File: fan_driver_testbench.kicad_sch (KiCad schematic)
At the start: 6 parts, among them Q5 BTS141

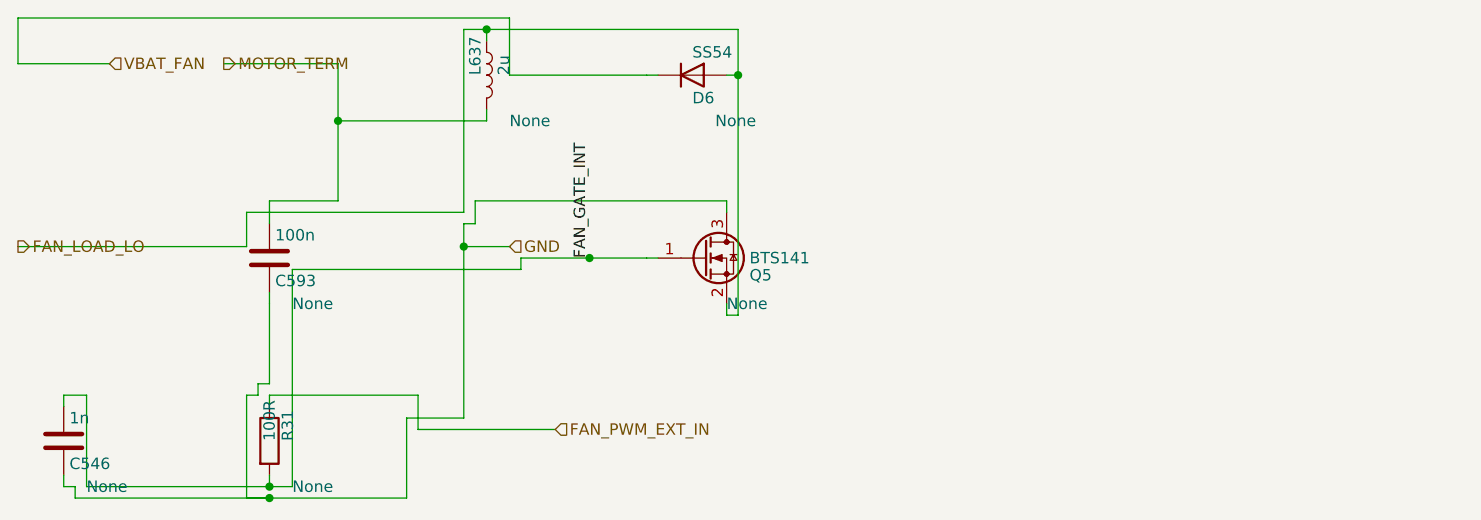
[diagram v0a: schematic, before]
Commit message: refactoring
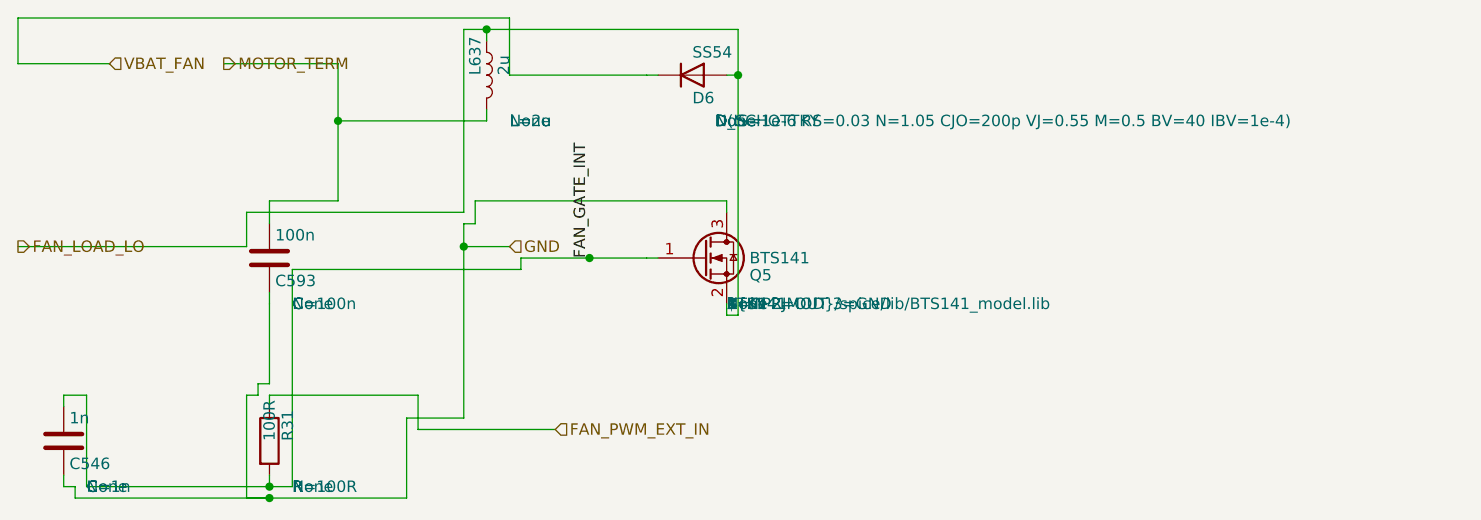
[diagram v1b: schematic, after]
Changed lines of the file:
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@@
+			)
+		)
+		(property "Sim.Device" "R"
+			(at 34.29 53.3399 0)
+			(effects
+				(font
+					(size 1.27 1.27)
+				)
+				(justify left)
+			)
+		)
+		(property "Sim.Params" "R=100R"
+			(at 34.29 53.3399 0)
+			(effects
+				(font
+					(size 1.27 1.27)
+				)
+				(justify left)
 			)
 		)
@@
 		(instances
 			(project "climate_control_niva_travel"
-				(path "/769b9906-d389-4980-b175-619cd77c101f"
+				(path "/04e9baa8-05c1-4d46-8e7f-66f0ccb7f2e0"
 					(reference "R31")
 					(unit 1)
@@
 			)
 		)
+		(property "Sim.Device" "C"
+			(at 11.43 53.3399 0)
+			(effects
+				(font
+					(size 1.27 1.27)
+				)
+				(justify left)
+			)
+		)
+		(property "Sim.Params" "C=1n"
+			(at 11.43 53.3399 0)
+			(effects
+				(font
+					(size 1.27 1.27)
+				)
+				(justify left)
+			)
+		)
 		(pin "1"
 		)
@@
 		(instances
 			(project "climate_control_niva_travel"
-				(path "/769b9906-d389-4980-b175-619cd77c101f"
+				(path "/04e9baa8-05c1-4d46-8e7f-66f0ccb7f2e0"
 					(reference "C546")
 					(unit 1)
@@
 			)
 		)
+		(property "Sim.Device" "X"
+			(at 82.55 33.0199 0)
+			(effects
+				(font
+					(size 1.27 1.27)
+				)
+				(justify left)
+			)
+		)
+		(property "Sim.Name" "BTS141"
+			(at 82.55 33.0199 0)
+			(effects
+				(font
+					(size 1.27 1.27)
+				)
+				(justify left)
+			)
+		)
+		(property "Sim.Library" "${KIPRJMOD}/spice/lib/BTS141_model.lib"
+			(at 82.55 33.0199 0)
+			(effects
+				(font
+					(size 1.27 1.27)
+				)
+				(justify left)
+			)
+		)
+		(property "Sim.Pins" "1=IN 2=OUT 3=GND"
+			(at 82.55 33.0199 0)
+			(effects
+				(font
+					(size 1.27 1.27)
+				)
+				(justify left)
+			)
+		)
+		(property "Sim.Enable" "1"
+			(at 82.55 33.0199 0)
+			(effects
+				(font
+					(size 1.27 1.27)
+				)
+				(justify left)
+			)
+		)
 		(pin "1"
 		)
@@
 		(instances
 			(project "climate_control_niva_travel"
-				(path "/769b9906-d389-4980-b175-619cd77c101f"
+				(path "/04e9baa8-05c1-4d46-8e7f-66f0ccb7f2e0"
 					(reference "Q5")
 					(unit 1)
@@
 			)
 		)
+		(property "Sim.Device" "D"
+			(at 81.28 12.6999 0)
+			(effects
+				(font
+					(size 1.27 1.27)
+				)
+				(justify left)
+			)
+		)
+		(property "Sim.Model" "D_SCHOTTKY"
+			(at 81.28 12.6999 0)
+			(effects
+				(font
+					(size 1.27 1.27)
+				)
+				(justify left)
+			)
+		)
+		(property "Sim.Params" "D(IS=1e-6 RS=0.03 N=1.05 CJO=200p VJ=0.55 M=0.5 BV=40 IBV=1e-4)"
+			(at 81.28 12.6999 0)
+			(effects
+				(font
+					(size 1.27 1.27)
+				)
+				(justify left)
+			)
+		)
 		(pin "1"
 		)
@@
 		(instances
 			(project "climate_control_niva_travel"
-				(path "/769b9906-d389-4980-b175-619cd77c101f"
+				(path "/04e9baa8-05c1-4d46-8e7f-66f0ccb7f2e0"
 					(reference "D6")
 					(unit 1)
@@
 			)
 		)
+		(property "Sim.Device" "L"
+			(at 58.42 12.6999 0)
+			(effects
+				(font
+					(size 1.27 1.27)
+				)
+				(justify left)
+			)
+		)
+		(property "Sim.Params" "L=2u"
+			(at 58.42 12.6999 0)
+			(effects
+				(font
+					(size 1.27 1.27)
+				)
+				(justify left)
+			)
+		)
 		(pin "1"
 		)
@@
 		(instances
 			(project "climate_control_niva_travel"
-				(path "/769b9906-d389-4980-b175-619cd77c101f"
+				(path "/04e9baa8-05c1-4d46-8e7f-66f0ccb7f2e0"
 					(reference "L637")
 					(unit 1)
@@
 			)
 		)
+		(property "Sim.Device" "C"
+			(at 34.29 33.0199 0)
+			(effects
+				(font
+					(size 1.27 1.27)
+				)
+				(justify left)
+			)
+		)
+		(property "Sim.Params" "C=100n"
+			(at 34.29 33.0199 0)
+			(effects
+				(font
+					(size 1.27 1.27)
+				)
+				(justify left)
+			)
+		)
 		(pin "1"
 		)
@@
 		(instances
 			(project "climate_control_niva_travel"
-				(path "/769b9906-d389-4980-b175-619cd77c101f"
+				(path "/04e9baa8-05c1-4d46-8e7f-66f0ccb7f2e0"
 					(reference "C593")
 					(unit 1)
@@
 	(junction
 		(at 31.75 53.34)
-		(diameter 0)
+		(diameter 0.0000)
 		(color 0 0 0 0)
 	)
 	(junction
 		(at 83.82 7.62)
-		(diameter 0)
+		(diameter 0.0000)
 		(color 0 0 0 0)
 	)
 	(junction
 		(at 55.88 2.54)
-		(diameter 0)
+		(diameter 0.0000)
 		(color 0 0 0 0)
 	)
 	(junction
 		(at 39.37 12.7)
-		(diameter 0)
+		(diameter 0.0000)
 		(color 0 0 0 0)
 	)
 	(junction
 		(at 53.34 26.67)
-		(diameter 0)
+		(diameter 0.0000)
 		(color 0 0 0 0)
 	)
 	(junction
 		(at 31.75 54.61)
-		(diameter 0)
+		(diameter 0.0000)
 		(color 0 0 0 0)
 	)
 	(junction
 		(at 67.31 27.94)
-		(diameter 0)
+		(diameter 0.0000)
 		(color 0 0 0 0)
 	)
